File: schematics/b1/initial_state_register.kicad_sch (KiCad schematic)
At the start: 13 parts, among them SW4 SW_DIP_x08, U3 74HC165

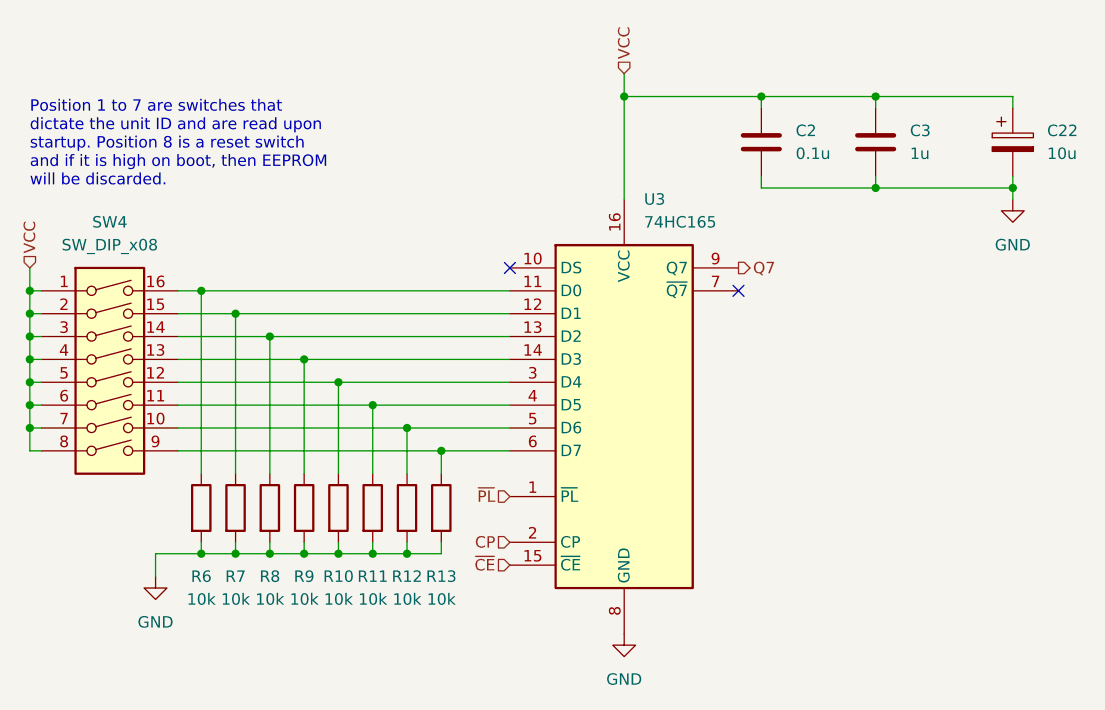
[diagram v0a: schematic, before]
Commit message: Added diode to prevent ISR from sinking other SPI MISO signals.
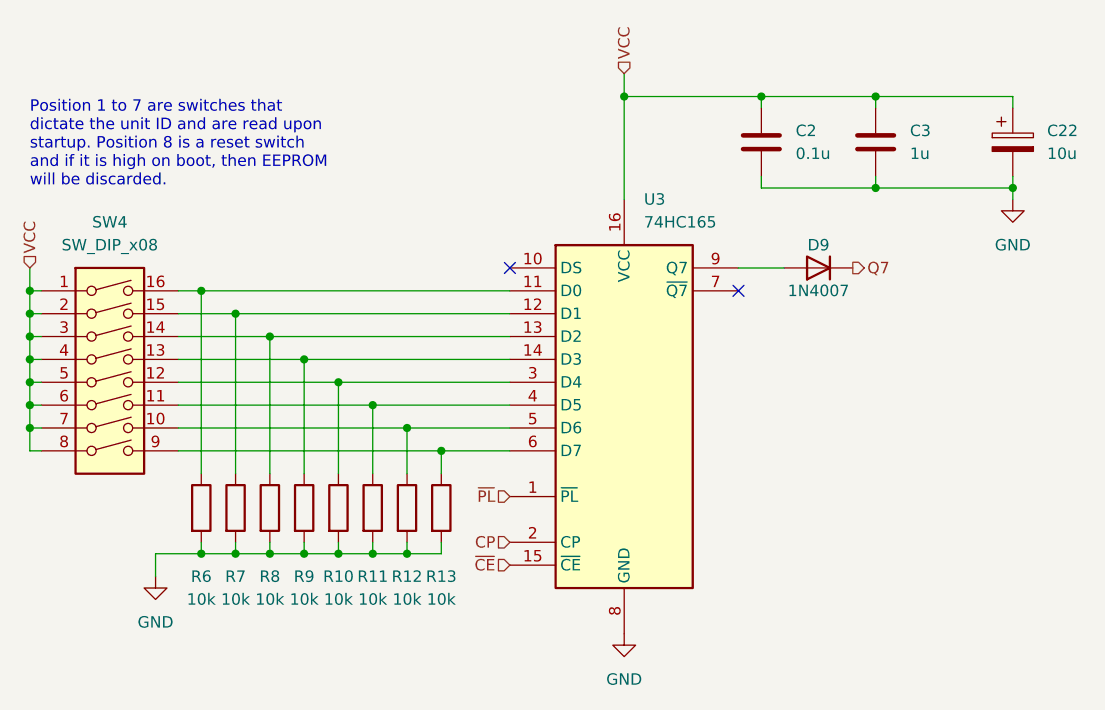
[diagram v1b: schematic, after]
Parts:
- added D9: 1N4007, Diode_THT:D_DO-41_SOD81_P10.16mm_Horizontal, symbol Diode:1N4007
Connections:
- net Q7: now also D9.1 (K); no longer U3.9 (Q7)
- new net: D9.2 (A), U3.9 (Q7)
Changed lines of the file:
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@@
+    (stroke (width 0) (type default))
+  )
+  (wire (pts (xy 134.62 50.8) (xy 129.54 50.8))
     (stroke (width 0) (type default))
   )
@@
     (effects (font (size 1.27 1.27)) (justify right))
   )
-  (hierarchical_label "Q7" (shape output) (at 129.54 50.8 0) (fields_autoplaced)
+  (hierarchical_label "Q7" (shape output) (at 142.24 50.8 0) (fields_autoplaced)
     (effects (font (size 1.27 1.27)) (justify left))
   )
@@
         )
       )
+    )
+  )
+  (symbol (lib_id "Diode:1N4007") (at 138.43 50.8 180) (unit 1)
+    (in_bom yes) (on_board yes) (dnp no)
+    (property "Reference" "D9" (at 138.43 48.26 0)
+      (effects (font (size 1.27 1.27)))
+    )
+    (property "Value" "1N4007" (at 138.43 53.34 0)
+      (effects (font (size 1.27 1.27)))
+    )
+    (property "Footprint" "Diode_THT:D_DO-41_SOD81_P10.16mm_Horizontal" (at 138.43 46.355 0)
+      (effects (font (size 1.27 1.27)) hide)
+    )
+    (property "Datasheet" "http://www.vishay.com/docs/88503/1n4001.pdf" (at 138.43 50.8 0)
+      (effects (font (size 1.27 1.27)) hide)
+    )
+    (property "Sim.Device" "D" (at 138.43 50.8 0)
+      (effects (font (size 1.27 1.27)) hide)
+    )
+    (property "Sim.Pins" "1=K 2=A" (at 138.43 50.8 0)
+      (effects (font (size 1.27 1.27)) hide)
+    )
+    (pin "2")
+    (pin "1")
+    (instances
+      (project "b1"
+        (path "/d6142fa5-2354-4512-9919-37616259c364/15951702-f191-4c4b-b68c-efdb5de618b5"
+          (reference "D9") (unit 1)
+        )
+      )

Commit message: Updated schematic to reflect manually shifting in ISR.
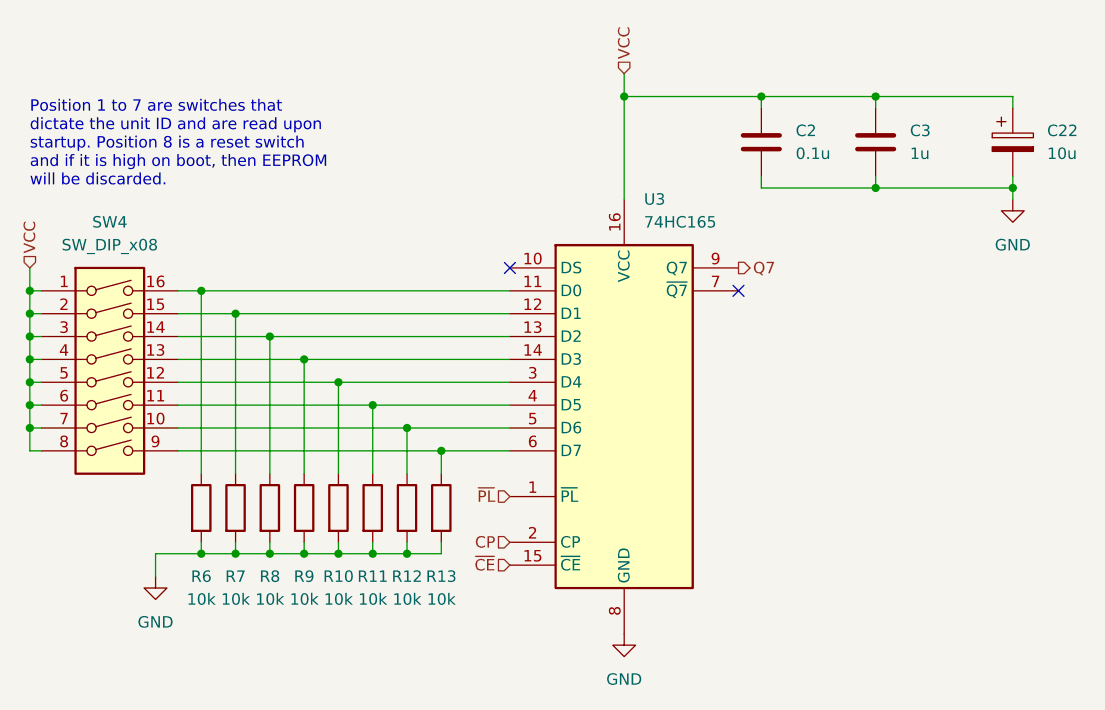
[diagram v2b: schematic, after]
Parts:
- removed D9: 1N4007, Diode_THT:D_DO-41_SOD81_P10.16mm_Horizontal, symbol Diode:1N4007
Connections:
- net Q7: now also U3.9 (Q7)
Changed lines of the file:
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@@
-    (stroke (width 0) (type default))
-  )
-  (wire (pts (xy 134.62 50.8) (xy 129.54 50.8))
     (stroke (width 0) (type default))
   )
@@
     (effects (font (size 1.27 1.27)) (justify right))
   )
-  (hierarchical_label "Q7" (shape output) (at 142.24 50.8 0) (fields_autoplaced)
+  (hierarchical_label "Q7" (shape output) (at 129.54 50.8 0) (fields_autoplaced)
     (effects (font (size 1.27 1.27)) (justify left))
   )
@@
         )
       )
-    )
-  )
-  (symbol (lib_id "Diode:1N4007") (at 138.43 50.8 180) (unit 1)
-    (in_bom yes) (on_board yes) (dnp no)
-    (property "Reference" "D9" (at 138.43 48.26 0)
-      (effects (font (size 1.27 1.27)))
-    )
-    (property "Value" "1N4007" (at 138.43 53.34 0)
-      (effects (font (size 1.27 1.27)))
-    )
-    (property "Footprint" "Diode_THT:D_DO-41_SOD81_P10.16mm_Horizontal" (at 138.43 46.355 0)
-      (effects (font (size 1.27 1.27)) hide)
-    )
-    (property "Datasheet" "http://www.vishay.com/docs/88503/1n4001.pdf" (at 138.43 50.8 0)
-      (effects (font (size 1.27 1.27)) hide)
-    )
-    (property "Sim.Device" "D" (at 138.43 50.8 0)
-      (effects (font (size 1.27 1.27)) hide)
-    )
-    (property "Sim.Pins" "1=K 2=A" (at 138.43 50.8 0)
-      (effects (font (size 1.27 1.27)) hide)
-    )
-    (pin "2")
-    (pin "1")
-    (instances
-      (project "b1"
-        (path "/d6142fa5-2354-4512-9919-37616259c364/15951702-f191-4c4b-b68c-efdb5de618b5"
-          (reference "D9") (unit 1)
-        )
-      )
